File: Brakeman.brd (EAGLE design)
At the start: 25.3 x 34.5 mm, 11 parts

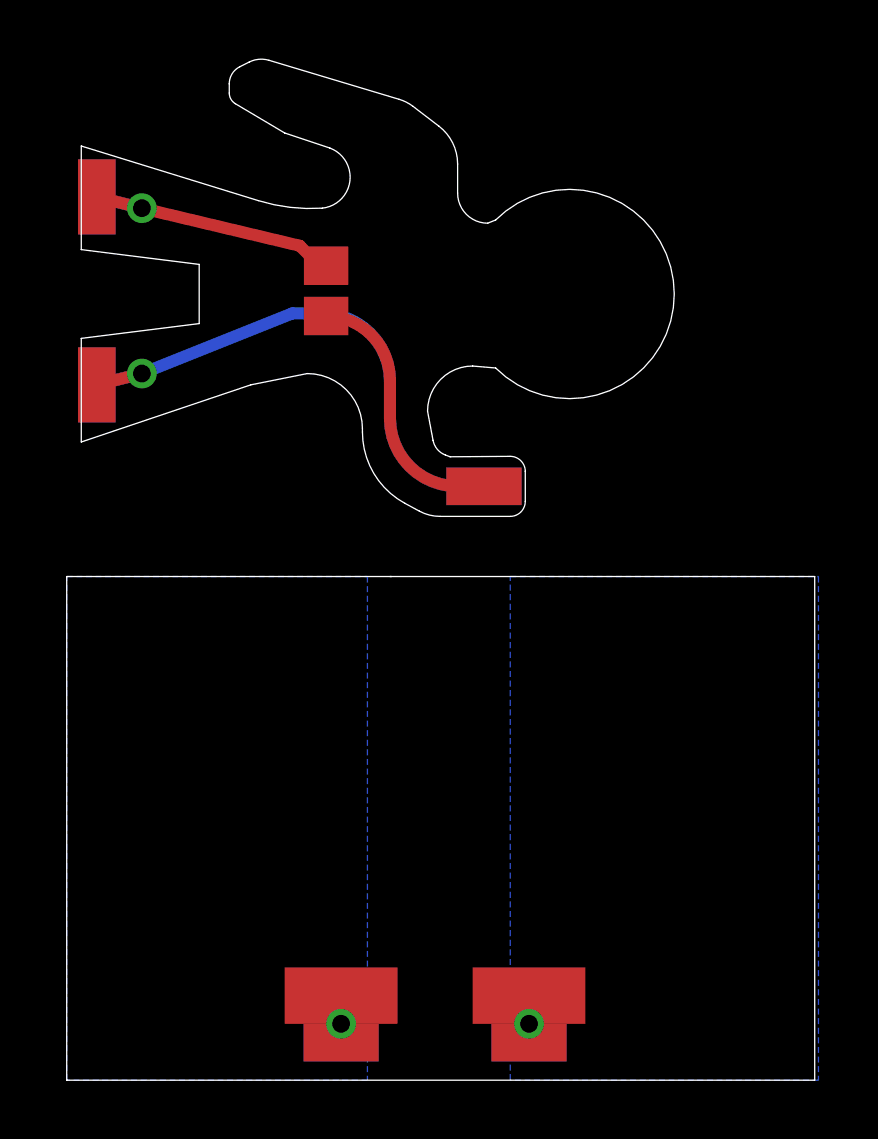
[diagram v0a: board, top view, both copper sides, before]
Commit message: 1.0
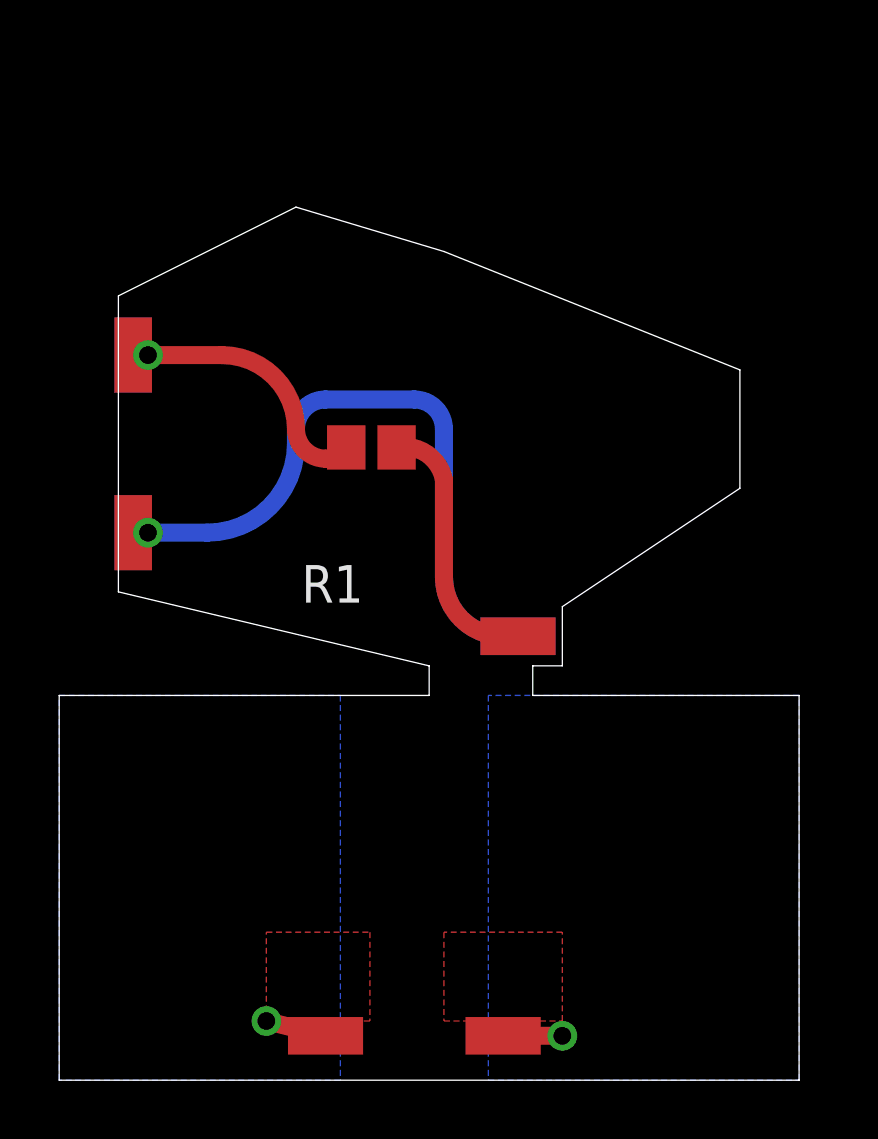
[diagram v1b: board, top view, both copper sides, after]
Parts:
- removed PAD10, PAD11, PAD12, PAD14, PAD20, PAD21, PAD23, PAD24: (no value), wirepad:SMD1.27-2.54
- added PAD3, PAD4, PAD5, PAD6, PAD7, PAD8: (no value), wirepad:SMD1.27-2.54
- moved PAD1 15.0 mm to (15.5, 15.0), flipped to the top, turned to 270 degrees
- moved PAD2 13.7 mm to (15.5, 15.0)
- moved R1 5.51 mm to (10.6, 21.4), turned to 180 degrees
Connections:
- removed net N$3: PAD14.1, R1.1
- new net N$2: PAD1.1, R1.1
- net N: now also PAD4.1, PAD6.1, PAD8.1; no longer PAD20.1, PAD21.1, PAD23.1, PAD24.1
- net S: now also PAD3.1, PAD5.1, PAD7.1; no longer PAD1.1, PAD10.1, PAD11.1, PAD12.1
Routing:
- net N$2: track 0.00 -> 8.55 mm
- net N$3: track 8.48 -> 0.00 mm
- net N: track 19.5 -> 23.5 mm
- added copper zone on layer 1, net N
- added copper zone on layer 1, net S
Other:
- board size 25.3 x 34.5 mm -> 25 x 29.5 mm
- board text added: "2012.01"
- board text removed: "2012.04"
- board text removed: "Add"
- board text removed: "DCC"
- board text removed: "here"
- board text removed: "weight"
